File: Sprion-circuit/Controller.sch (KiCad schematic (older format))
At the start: 26 parts, among them J2 Conn_01x04_Female, J6 Conn_01x04_Female, Q3 IRFML8244, Q4 RUE002N02, SW2 SW_Push, SW3 SW_Push, SW4 SW_Push, U3 STM32F405RGTx

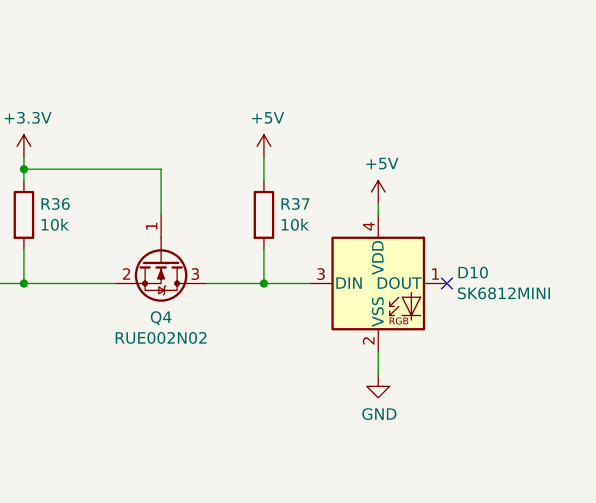
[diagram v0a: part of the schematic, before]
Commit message: add fix feat: でけたー（コミットしてなくてごめん）
ベタ塗、配線、再配置等
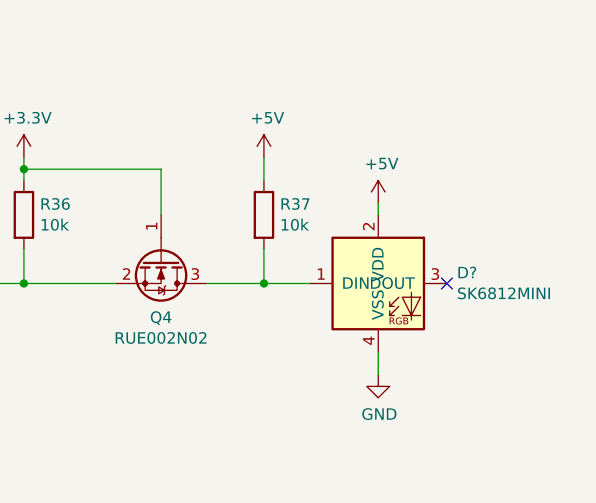
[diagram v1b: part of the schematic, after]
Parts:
- removed D10: SK6812MINI, LED_SMD:LED_SK6812MINI_PLCC4_3.5x3.5mm_P1.75mm, symbol LED:SK6812MINI
- added D?: SK6812MINI, symbol Sprion-circuit:SK6812MINI
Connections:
- net +5V: now also D?.2 (VDD)
- net GND: now also D?.4 (VSS)
- net at Q4.3 (D), R37.2: now also D?.1 (DIN)
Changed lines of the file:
@@
 $Descr A4 11693 8268
 encoding utf-8
-Sheet 5 6
+Sheet 4 6
 Title ""
 Date ""
@@
 	1350 2950 1350 3350
 Connection ~ 1350 3350
-$Comp
-L LED:SK6812MINI D10
-U 1 1 60EFAFD7
-P 10000 5300
-F 0 "D10" H 10344 5346 50  0000 L CNN
-F 1 "SK6812MINI" H 10344 5255 50  0000 L CNN
-F 2 "LED_SMD:LED_SK6812MINI_PLCC4_3.5x3.5mm_P1.75mm" H 10050 5000 50  0001 L TNN
-F 3 "https://cdn-shop.adafruit.com/product-files/2686/SK6812MINI_REV.01-1-2.pdf" H 10100 4925 50  0001 L TNN
-	1    10000 5300
-	1    0    0    -1
-$EndComp
 Wire Wire Line
 	2300 4650 2550 4650
@@
 	0    1    1    0
 $EndComp
+$Comp
+L Sprion-circuit:SK6812MINI D?
+U 1 1 61C04E87
+P 10000 5300
+F 0 "D?" H 10344 5346 50  0000 L CNN
+F 1 "SK6812MINI" H 10344 5255 50  0000 L CNN
+F 2 "" H 10000 5750 50  0001 C CNN
+F 3 "" H 10000 5750 50  0001 C CNN
+	1    10000 5300
+	1    0    0    -1
+$EndComp
 $EndSCHEMATC
